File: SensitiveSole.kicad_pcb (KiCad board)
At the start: 2 copper layers, 33 x 33 mm, 28 parts, among them J1 Conn_01x24, U1 CD74HC4067SM, U2 CD74HC4067SM

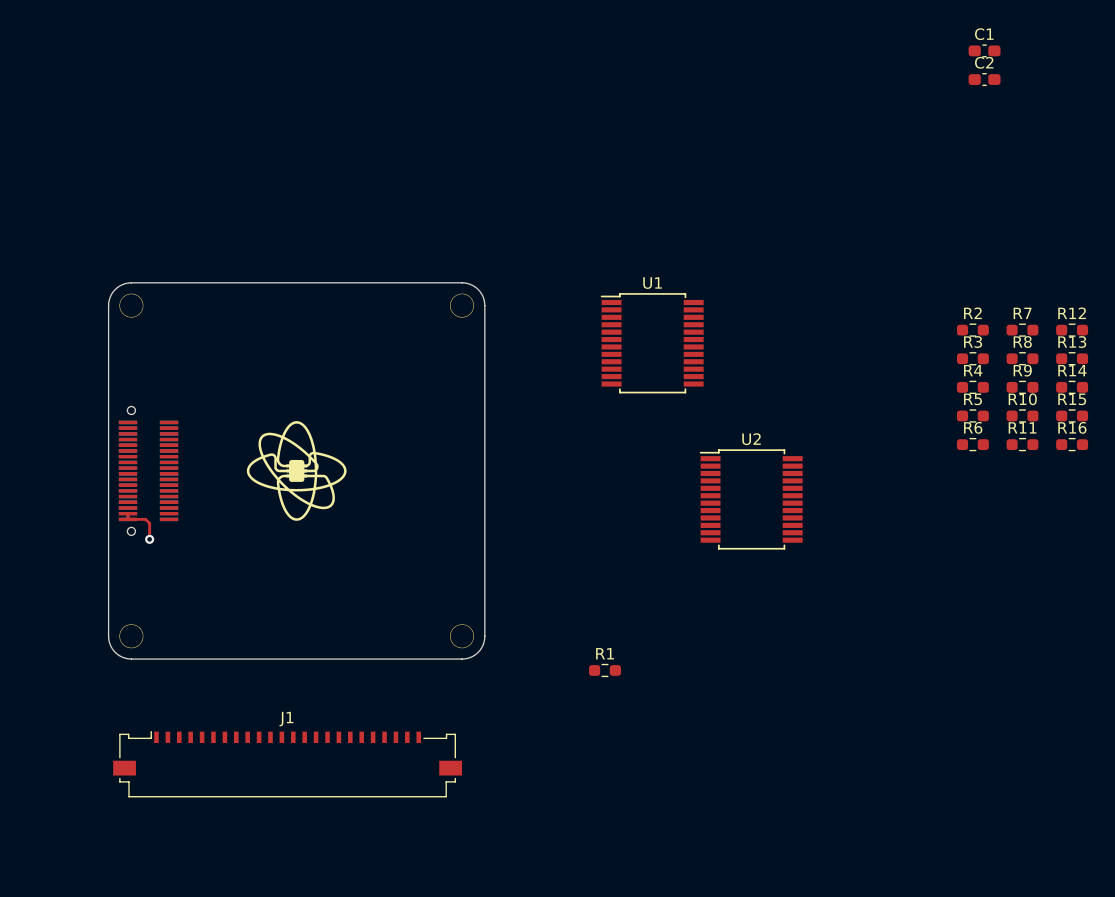
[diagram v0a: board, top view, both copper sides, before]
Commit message: base clean
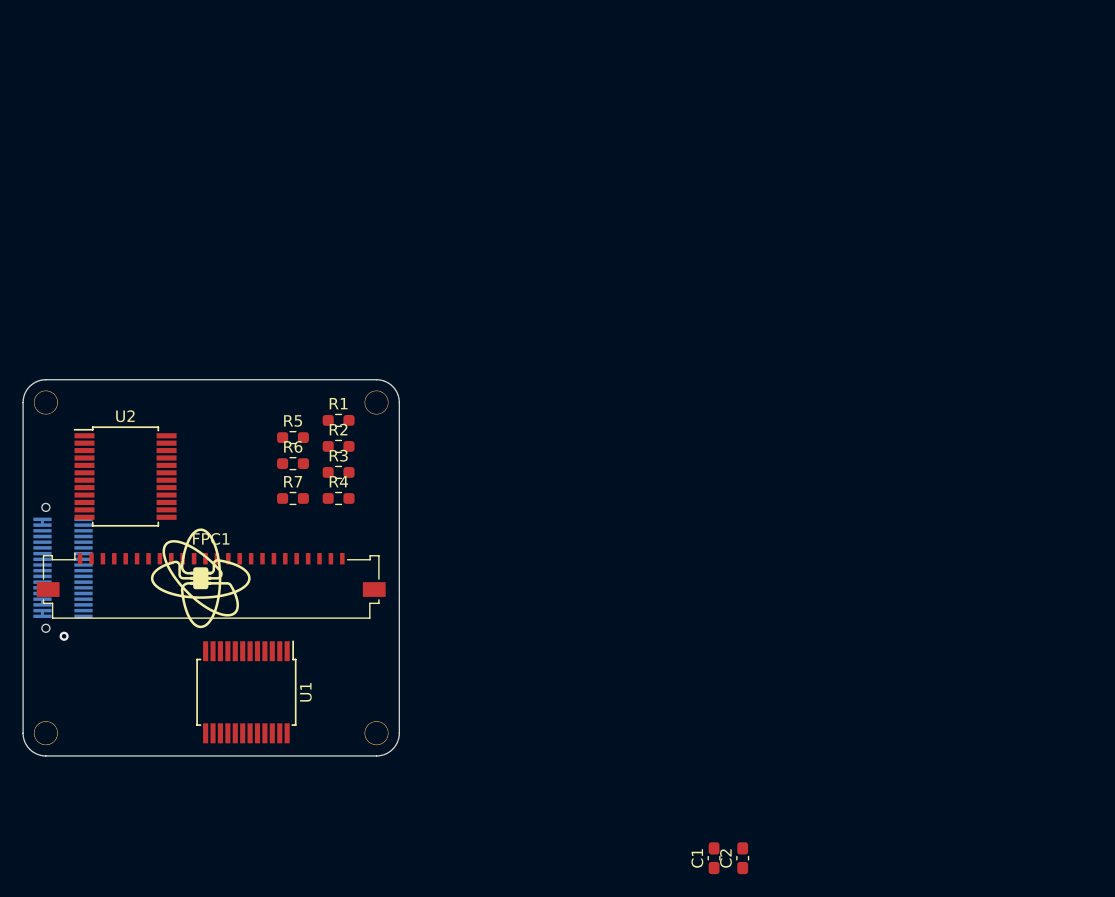
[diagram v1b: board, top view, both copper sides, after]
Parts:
- removed R10, R11, R12, R13, R14, R15, R16, R8, R9: 10k, Resistor_SMD:R_0603_1608Metric_Pad0.98x0.95mm_HandSolder
- removed TOP_DF12: DF12-36NOLEGS-FEMALE, MovuinoESP8266:DF12-36-DP-NL-noPad
- moved C1 74.7 mm to (180.6, 129.0), turned to 90 degrees
- moved C2 71.5 mm to (183.1, 129.0), turned to 90 degrees
- moved R7 65.7 mm to (143.7, 97.4)
- moved R5 59.7 mm to (143.7, 92.1)
- moved R6 59.7 mm to (143.7, 94.4)
- moved R2 56.6 mm to (147.7, 92.9)
- moved R3 56.5 mm to (147.7, 95.1)
- moved R4 56.5 mm to (147.7, 97.4)
- moved U2 55.0 mm to (129.0, 95.5)
- moved U1 47.0 mm to (139.6, 114.4), turned to -90 degrees
- moved R1 32.0 mm to (147.7, 90.6)
- moved FPC1 17.0 mm to (136.5, 103.6)
- moved U$8 12.6 mm to (135.2, 104.1)
- moved ? 11.3 mm to (151.0, 118.0)
- moved ? 11.3 mm to (122.0, 89.0)
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- renumbered J1 to FPC1
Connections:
- BOTTOM_DF12 pad 1: /IO36 -> unconnected-(BOTTOM_DF12-Pad1)
- BOTTOM_DF12 pad 11: /IO35 -> unconnected-(BOTTOM_DF12-Pad11)
- BOTTOM_DF12 pad 25: /IO15 -> unconnected-(BOTTOM_DF12-Pad25)
- BOTTOM_DF12 pad 29: /IO13 -> unconnected-(BOTTOM_DF12-Pad29)
- BOTTOM_DF12 pad 3: /IO38 -> unconnected-(BOTTOM_DF12-Pad3)
- BOTTOM_DF12 pad 31: /IO4 -> unconnected-(BOTTOM_DF12-Pad31)
- BOTTOM_DF12 pad 35: /GPIO2 -> /IO2
- BOTTOM_DF12 pad 7: /IO34 -> unconnected-(BOTTOM_DF12-Pad7)
- BOTTOM_DF12 pad 9: /IO37 -> unconnected-(BOTTOM_DF12-Pad9)
- FPC1 pad 10: unconnected-(J1-Pin_10-Pad10) -> /ROW8
- FPC1 pad 11: unconnected-(J1-Pin_11-Pad11) -> /ROW9
- FPC1 pad 12: unconnected-(J1-Pin_12-Pad12) -> /ROW10
- FPC1 pad 13: unconnected-(J1-Pin_13-Pad13) -> /ROW11
- FPC1 pad 14: unconnected-(J1-Pin_14-Pad14) -> /ROW12
- FPC1 pad 15: unconnected-(J1-Pin_15-Pad15) -> /ROW13
- FPC1 pad 16: unconnected-(J1-Pin_16-Pad16) -> /ROW14
- FPC1 pad 17: unconnected-(J1-Pin_17-Pad17) -> /COL6
- FPC1 pad 18: unconnected-(J1-Pin_18-Pad18) -> /COL5
- FPC1 pad 19: unconnected-(J1-Pin_19-Pad19) -> /COL4
- FPC1 pad 2: unconnected-(J1-Pin_2-Pad2) -> /ROW0
- FPC1 pad 20: unconnected-(J1-Pin_20-Pad20) -> /COL3
- FPC1 pad 21: unconnected-(J1-Pin_21-Pad21) -> /COL2
- FPC1 pad 22: unconnected-(J1-Pin_22-Pad22) -> /COL1
- FPC1 pad 23: unconnected-(J1-Pin_23-Pad23) -> /COL0
- FPC1 pad 3: unconnected-(J1-Pin_3-Pad3) -> /ROW1
- FPC1 pad 4: unconnected-(J1-Pin_4-Pad4) -> /ROW2
- FPC1 pad 5: unconnected-(J1-Pin_5-Pad5) -> /ROW3
- FPC1 pad 6: unconnected-(J1-Pin_6-Pad6) -> /ROW4
- FPC1 pad 7: unconnected-(J1-Pin_7-Pad7) -> /ROW5
- FPC1 pad 8: unconnected-(J1-Pin_8-Pad8) -> /ROW6
- FPC1 pad 9: unconnected-(J1-Pin_9-Pad9) -> /ROW7
- U1 pad 1: /IO25 -> /IO39
- U1 pad 10: /IO33 -> /IO32
- U1 pad 11: /IO32 -> /IO33
- U1 pad 13: /IO27 -> /IO26
- U1 pad 14: /IO26 -> /IO25
- U1 pad 16: /COL15 -> unconnected-(U1-I15-Pad16)
- U1 pad 17: /COL14 -> unconnected-(U1-I14-Pad17)
- U1 pad 18: /COL13 -> unconnected-(U1-I13-Pad18)
- U1 pad 19: /COL12 -> unconnected-(U1-I12-Pad19)
- U1 pad 2: /COL7 -> unconnected-(U1-I7-Pad2)
- U1 pad 20: /COL11 -> unconnected-(U1-I11-Pad20)
- U1 pad 21: /COL10 -> unconnected-(U1-I10-Pad21)
- U1 pad 22: /COL9 -> unconnected-(U1-I9-Pad22)
- U1 pad 23: /COL8 -> unconnected-(U1-I8-Pad23)
- U2 pad 1: /IO12 -> /IO2
- U2 pad 10: /IO13 -> /IO27
- U2 pad 11: /IO4 -> /IO14
- U2 pad 13: /IO14 -> /IO5
- U2 pad 14: /IO15 -> /IO12
- U2 pad 16: /ROW15 -> unconnected-(U2-I15-Pad16)
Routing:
- net GND: track 4.25 -> 0.50 mm
- net +5V: track 0.00 -> 0.50 mm
- net +3.3V: track 0.00 -> 0.50 mm
